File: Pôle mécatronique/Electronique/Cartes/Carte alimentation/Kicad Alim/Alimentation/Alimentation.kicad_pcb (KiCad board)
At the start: 2 copper layers, 65 x 85 mm, 27 parts, among them J1 Conn_01x04, J2 Conn_01x04, J3 Conn_01x04, J4 Conn_01x05, J5 Conn_01x05, J6 Conn_02x03_Odd_Even, J7 Conn_02x10_Odd_Even, J8 24V in, J9 24V out, K1 G5LE-1, Q1 BD135, SW1 SW_DPDT_x2, U1 TSR_2-2450, U2 TSR_2-2450, U3 TSR_2-24120

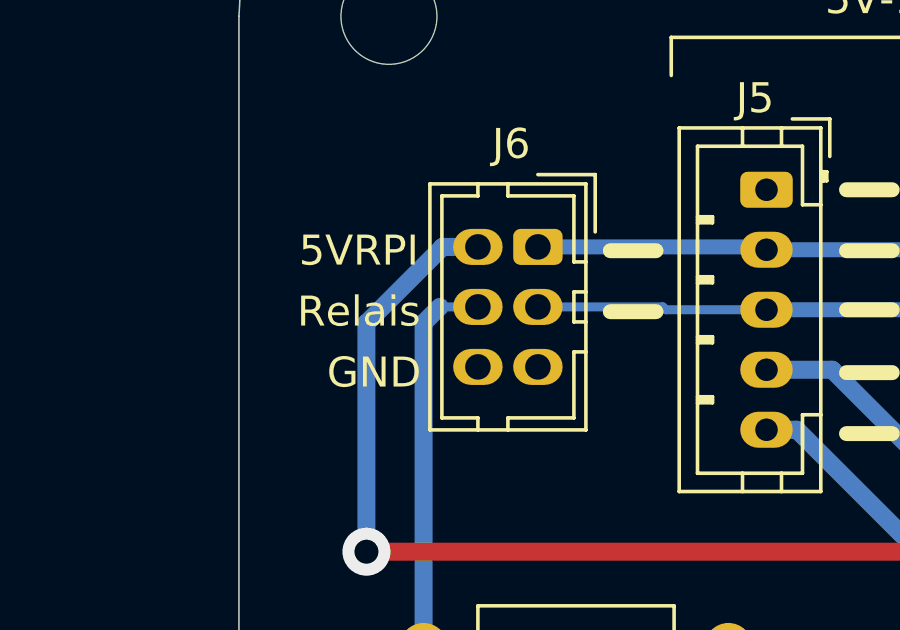
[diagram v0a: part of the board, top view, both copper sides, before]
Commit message: Update HAT
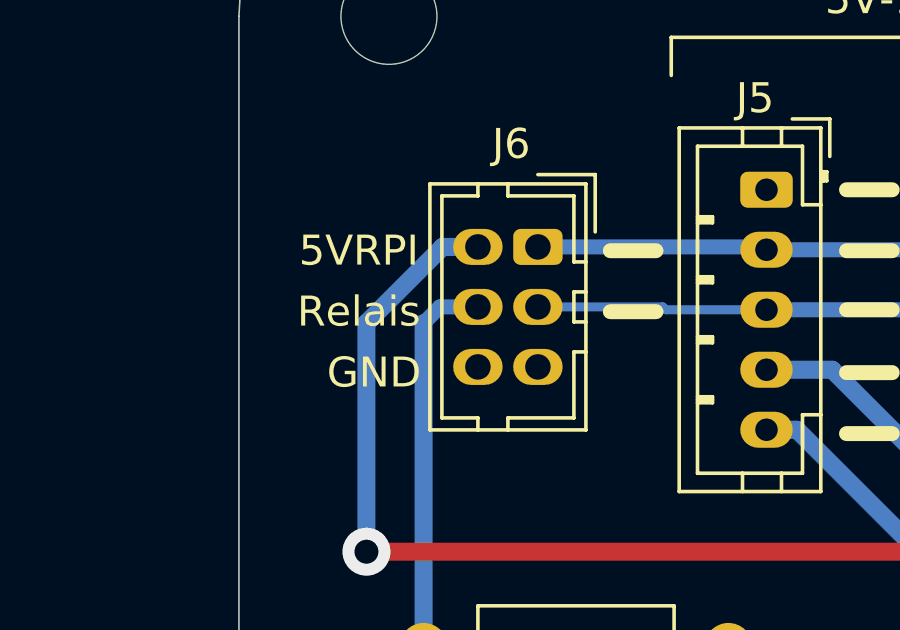
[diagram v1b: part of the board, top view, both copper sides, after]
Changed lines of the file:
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@@
   (segment (start 120.142 72.898) (end 120.142 67.183) (width 0.6) (layer "B.Cu") (net 7))
   (segment (start 118.3645 59.4355) (end 113.792 54.863) (width 0.6) (layer "B.Cu") (net 7))
-  (segment (start 94.647 50.133) (end 95.917 50.133) (width 0.3) (layer "B.Cu") (net 8))
-  (segment (start 94.107 50.673) (end 94.647 50.133) (width 0.6) (layer "B.Cu") (net 8))
   (segment (start 94.107 61.468) (end 94.107 50.673) (width 0.6) (layer "B.Cu") (net 8))
+  (segment (start 94.647 50.133) (end 94.107 50.673) (width 0.5) (layer "B.Cu") (net 8))
+  (segment (start 95.917 50.133) (end 94.647 50.133) (width 0.5) (layer "B.Cu") (net 8))
   (segment (start 135.382 58.293) (end 92.202 58.293) (width 0.6) (layer "F.Cu") (net 9))
   (via (at 135.382 58.293) (size 1.6) (drill 0.8) (layers "F.Cu" "B.Cu") (net 9))
